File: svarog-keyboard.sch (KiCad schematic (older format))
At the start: 311 parts, among them J1 AVR-ISP-6, J10 I2C, J2 Conn_01x08_Male, J3 I2C, J4 I2C, J5 I2C, J6 I2C, J7 I2C, J8 I2C, J9 I2C, K1 KEYSW, K10 KEYSW, K11 KEYSW, K12 KEYSW, K13 KEYSW, K13-1 KEYSW, K14 KEYSW, K14-1 KEYSW, K14-2 KEYSW, K15 KEYSW, K16 KEYSW, K17 KEYSW, K18 KEYSW, K19 KEYSW, K2 KEYSW, K20 KEYSW, K21 KEYSW, K3 KEYSW, K4 KEYSW, K5 KEYSW, K6 KEYSW, K7 KEYSW, K8 KEYSW, K9 KEYSW, SW1 SW_BOOT, SW2 SW_RESET, U1 ATmega32A-PU, U2 MCP23017_SP, U3 MCP23017_SP, U4 MCP23017_SP, Y1 Crystal

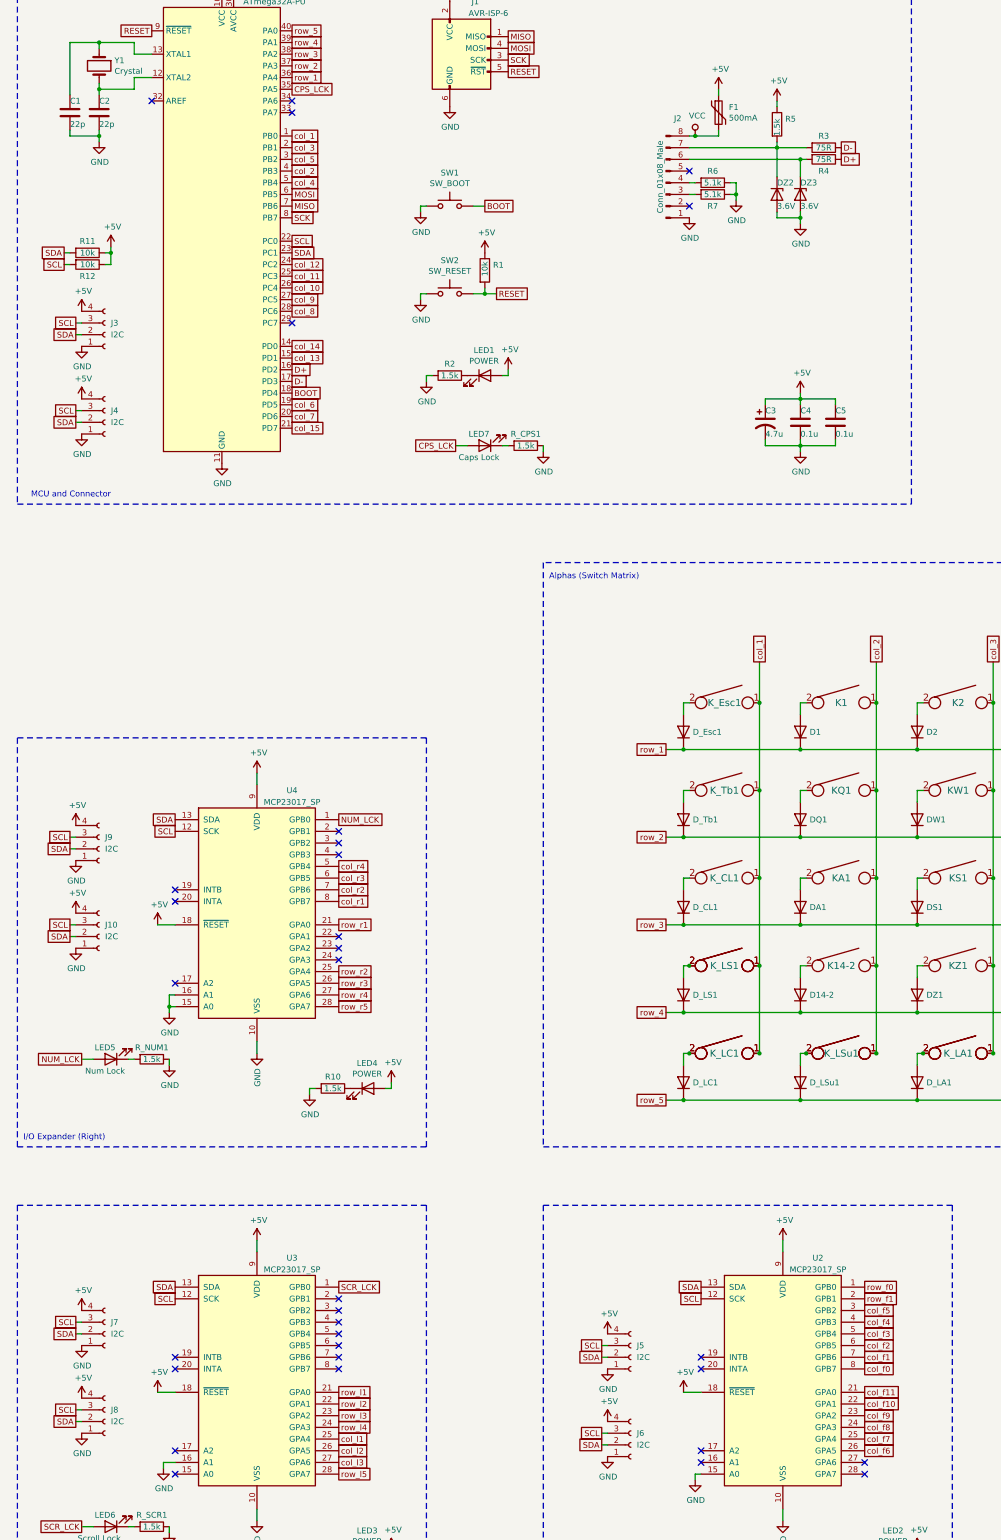
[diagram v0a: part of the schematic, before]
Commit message: Rev 0.1 [ALPHA] [UNTESTED]
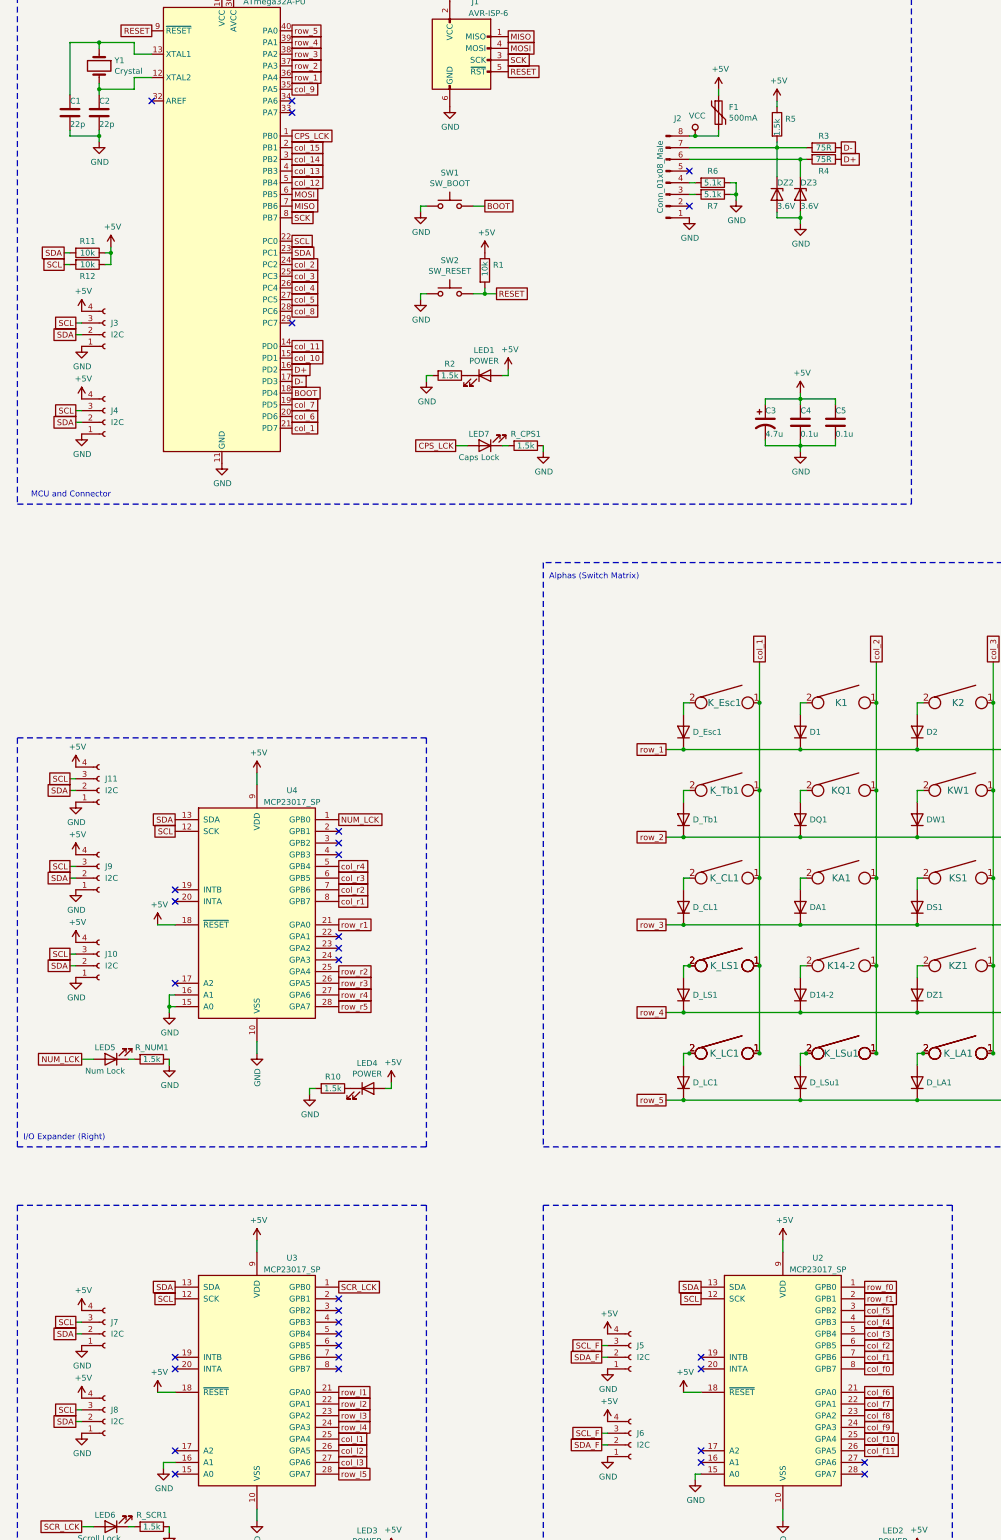
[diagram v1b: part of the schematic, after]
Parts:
- added J11: I2C, Connector_PinHeader_2.54mm:PinHeader_1x04_P2.54mm_Vertical, symbol Connector:Conn_01x04_Female
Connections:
- net +5V: now also J11.4 (Pin_4)
- net CPS_LCK: now also U1.1 (PB0); no longer U1.35 (PA5)
- net GND: now also J11.1 (Pin_1)
- net SCL: now also J11.3 (Pin_3); no longer J5.3 (Pin_3), J6.3 (Pin_3)
- net SDA: now also J11.2 (Pin_2); no longer J5.2 (Pin_2), J6.2 (Pin_2)
- net col_1: now also U1.21 (PD7); no longer U1.1 (PB0)
- net col_10: now also U1.15 (PD1); no longer U1.26 (PC4)
- net col_11: now also U1.14 (PD0); no longer U1.25 (PC3)
- net col_12: now also U1.5 (PB4); no longer U1.24 (PC2)
- net col_13: now also U1.4 (PB3); no longer U1.15 (PD1)
- net col_14: now also U1.3 (PB2); no longer U1.14 (PD0)
- net col_15: now also U1.2 (PB1); no longer U1.21 (PD7)
- net col_2: now also U1.24 (PC2); no longer U1.4 (PB3)
- net col_3: now also U1.25 (PC3); no longer U1.2 (PB1)
- net col_4: now also U1.26 (PC4); no longer U1.5 (PB4)
- net col_5: now also U1.27 (PC5); no longer U1.3 (PB2)
- net col_6: now also U1.20 (PD6); no longer U1.19 (PD5)
- net col_7: now also U1.19 (PD5); no longer U1.20 (PD6)
- net col_9: now also U1.35 (PA5); no longer U1.27 (PC5)
- net col_f10: now also U2.25 (GPA4); no longer U2.22 (GPA1)
- net col_f11: now also U2.26 (GPA5); no longer U2.21 (GPA0)
- net col_f6: now also U2.21 (GPA0); no longer U2.26 (GPA5)
- net col_f7: now also U2.22 (GPA1); no longer U2.25 (GPA4)
- net col_f8: now also U2.23 (GPA2); no longer U2.24 (GPA3)
- net col_f9: now also U2.24 (GPA3); no longer U2.23 (GPA2)
- new net SCL_F: J5.3 (Pin_3), J6.3 (Pin_3)
- new net SDA_F: J5.2 (Pin_2), J6.2 (Pin_2)
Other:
- moved on the sheet: J10, J9
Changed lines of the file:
@@
 Text GLabel 3350 1750 2    50   UnSpc ~ 0
 row_2
-Text GLabel 3350 2350 2    50   UnSpc ~ 0
+Text GLabel 3350 4850 2    50   UnSpc ~ 0
 col_1
-Text GLabel 3350 2450 2    50   UnSpc ~ 0
+Text GLabel 3350 3550 2    50   UnSpc ~ 0
 col_3
-Text GLabel 3350 2550 2    50   UnSpc ~ 0
+Text GLabel 3350 3750 2    50   UnSpc ~ 0
 col_5
 Text GLabel 3350 1450 2    50   UnSpc ~ 0
@@
 Text GLabel 3350 1850 2    50   UnSpc ~ 0
 row_1
+Text GLabel 3350 3450 2    50   UnSpc ~ 0
+col_2
+Text GLabel 3350 3650 2    50   UnSpc ~ 0
+col_4
+Text GLabel 3350 2550 2    50   UnSpc ~ 0
+col_14
 Text GLabel 3350 2650 2    50   UnSpc ~ 0
-col_2
+col_13
 Text GLabel 3350 2750 2    50   UnSpc ~ 0
-col_4
+col_12
 Text GLabel 3350 4150 2    50   UnSpc ~ 0
-col_14
+col_11
 Text GLabel 3350 4250 2    50   UnSpc ~ 0
-col_13
-Text GLabel 3350 3450 2    50   UnSpc ~ 0
-col_12
-Text GLabel 3350 3550 2    50   UnSpc ~ 0
-col_11
-Text GLabel 3350 3650 2    50   UnSpc ~ 0
 col_10
-Text GLabel 3350 3750 2    50   UnSpc ~ 0
+Text GLabel 3350 1950 2    50   UnSpc ~ 0
 col_9
 Text GLabel 3350 3850 2    50   UnSpc ~ 0
 col_8
+Text GLabel 3350 4650 2    50   UnSpc ~ 0
+col_7
+Text GLabel 3350 2450 2    50   UnSpc ~ 0
+col_15
 Text GLabel 3350 4750 2    50   UnSpc ~ 0
-col_7
-Text GLabel 3350 4850 2    50   UnSpc ~ 0
-col_15
-Text GLabel 3350 4650 2    50   UnSpc ~ 0
 col_6
 Wire Notes Line
@@
 Text GLabel 2350 8200 0    50   UnSpc ~ 0
 SDA
+Text GLabel 8250 13500 2    50   UnSpc ~ 0
+col_f10
+Text GLabel 8250 13600 2    50   UnSpc ~ 0
+col_f11
+Text GLabel 8250 13300 2    50   UnSpc ~ 0
+col_f8
+Text GLabel 8250 13400 2    50   UnSpc ~ 0
+col_f9
+Text GLabel 8250 13100 2    50   UnSpc ~ 0
+col_f6
 Text GLabel 8250 13200 2    50   UnSpc ~ 0
-col_f10
-Text GLabel 8250 13100 2    50   UnSpc ~ 0
-col_f11
-Text GLabel 8250 13400 2    50   UnSpc ~ 0
-col_f8
-Text GLabel 8250 13300 2    50   UnSpc ~ 0
-col_f9
-Text GLabel 8250 13600 2    50   UnSpc ~ 0
-col_f6
-Text GLabel 8250 13500 2    50   UnSpc ~ 0
 col_f7
 Text GLabel 8250 12500 2    50   UnSpc ~ 0
@@
 Wire Wire Line
 	1950 14250 2000 14250
-Text GLabel 3350 1950 2    50   UnSpc ~ 0
+Text GLabel 3350 2350 2    50   UnSpc ~ 0
 CPS_LCK
 Text GLabel 3750 8200 2    50   UnSpc ~ 0
@@
 $EndComp
 Text GLabel 6000 12800 0    50   UnSpc ~ 0
-SDA
+SDA_F
 Text GLabel 6000 12700 0    50   UnSpc ~ 0
-SCL
+SCL_F
 Wire Wire Line
 	6050 12700 6000 12700
@@
 	1    0    0    -1
 $EndComp
-Text GLabel 1450 8450 0    50   UnSpc ~ 0
+Text GLabel 1450 8700 0    50   UnSpc ~ 0
 SDA
-Text GLabel 1450 8350 0    50   UnSpc ~ 0
+Text GLabel 1450 8600 0    50   UnSpc ~ 0
 SCL
 Wire Wire Line
-	1500 8350 1450 8350
-Wire Wire Line
-	1500 8450 1450 8450
+	1500 8600 1450 8600
+Wire Wire Line
+	1500 8700 1450 8700
 $Comp
 L Connector:Conn_01x04_Female J9
 U 1 1 60AAE1B6
-P 1700 8450
-F 0 "J9" H 1750 8350 50  0000 L CNN
-F 1 "I2C" H 1750 8450 50  0000 L CNN
-F 2 "Connector_PinHeader_2.54mm:PinHeader_1x04_P2.54mm_Vertical" H 1700 8450 50  0001 C CNN
-F 3 "~" H 1700 8450 50  0001 C CNN
-	1    1700 8450
+P 1700 8700
+F 0 "J9" H 1750 8600 50  0000 L CNN
+F 1 "I2C" H 1750 8700 50  0000 L CNN
+F 2 "Connector_PinHeader_2.54mm:PinHeader_1x04_P2.54mm_Vertical" H 1700 8700 50  0001 C CNN
+F 3 "~" H 1700 8700 50  0001 C CNN
+	1    1700 8700
 	1    0    0    1
 $EndComp
@@
 L power:GND #PWR0152
 U 1 1 60AAE1BC
-P 1500 8550
-F 0 "#PWR0152" H 1500 8300 50  0001 C CNN
-F 1 "GND" H 1505 8377 50  0000 C CNN
-F 2 "" H 1500 8550 50  0001 C CNN
-F 3 "" H 1500 8550 50  0001 C CNN
-	1    1500 8550
+P 1500 8800
+F 0 "#PWR0152" H 1500 8550 50  0001 C CNN
+F 1 "GND" H 1505 8627 50  0000 C CNN
+F 2 "" H 1500 8800 50  0001 C CNN
+F 3 "" H 1500 8800 50  0001 C CNN
+	1    1500 8800
 	1    0    0    -1
 $EndComp
@@
 L power:+5V #PWR0153
 U 1 1 60AAE1C2
-P 1500 8250
-F 0 "#PWR0153" H 1500 8100 50  0001 C CNN
-F 1 "+5V" H 1515 8423 50  0000 C CNN
-F 2 "" H 1500 8250 50  0001 C CNN
-F 3 "" H 1500 8250 50  0001 C CNN
-	1    1500 8250
+P 1500 8500
+F 0 "#PWR0153" H 1500 8350 50  0001 C CNN
+F 1 "+5V" H 1515 8673 50  0000 C CNN
+F 2 "" H 1500 8500 50  0001 C CNN
+F 3 "" H 1500 8500 50  0001 C CNN
+	1    1500 8500
 	1    0    0    -1
 $EndComp
@@
 $EndComp
 Text GLabel 6000 13550 0    50   UnSpc ~ 0
-SDA
+SDA_F
 Text GLabel 6000 13450 0    50   UnSpc ~ 0
-SCL
+SCL_F
 Wire Wire Line
 	6050 13450 6000 13450
@@
 F 3 "" H 1550 13150 50  0001 C CNN
 	1    1550 13150
-	1    0    0    -1
-$EndComp
-Text GLabel 1450 9200 0    50   UnSpc ~ 0
-SDA
-Text GLabel 1450 9100 0    50   UnSpc ~ 0
-SCL
-Wire Wire Line
-	1500 9100 1450 9100
-Wire Wire Line
-	1500 9200 1450 9200
-$Comp
-L Connector:Conn_01x04_Female J10
-U 1 1 5E9D4282
-P 1700 9200
-F 0 "J10" H 1750 9100 50  0000 L CNN
-F 1 "I2C" H 1750 9200 50  0000 L CNN
-F 2 "Connector_PinHeader_2.54mm:PinHeader_1x04_P2.54mm_Vertical" H 1700 9200 50  0001 C CNN
-F 3 "~" H 1700 9200 50  0001 C CNN
-	1    1700 9200
-	1    0    0    1
-$EndComp
-$Comp
-L power:GND #PWR0161
-U 1 1 5E9D4288
-P 1500 9300
-F 0 "#PWR0161" H 1500 9050 50  0001 C CNN
-F 1 "GND" H 1505 9127 50  0000 C CNN
-F 2 "" H 1500 9300 50  0001 C CNN
-F 3 "" H 1500 9300 50  0001 C CNN
-	1    1500 9300
-	1    0    0    -1
-$EndComp
-$Comp
-L power:+5V #PWR0162
-U 1 1 5E9D428E
-P 1500 9000
-F 0 "#PWR0162" H 1500 8850 50  0001 C CNN
-F 1 "+5V" H 1515 9173 50  0000 C CNN
-F 2 "" H 1500 9000 50  0001 C CNN
-F 3 "" H 1500 9000 50  0001 C CNN
-	1    1500 9000
 	1    0    0    -1
 $EndComp
@@
 NoConn ~ 3750 8300
 NoConn ~ 3750 9200
+$Comp
+L power:+5V #PWR0162
+U 1 1 5E9D428E
+P 1500 9250
+F 0 "#PWR0162" H 1500 9100 50  0001 C CNN
+F 1 "+5V" H 1515 9423 50  0000 C CNN
+F 2 "" H 1500 9250 50  0001 C CNN
+F 3 "" H 1500 9250 50  0001 C CNN
+	1    1500 9250
+	1    0    0    -1
+$EndComp
+$Comp
+L power:GND #PWR0161
+U 1 1 5E9D4288
+P 1500 9550
+F 0 "#PWR0161" H 1500 9300 50  0001 C CNN
+F 1 "GND" H 1505 9377 50  0000 C CNN
+F 2 "" H 1500 9550 50  0001 C CNN
+F 3 "" H 1500 9550 50  0001 C CNN
+	1    1500 9550
+	1    0    0    -1
+$EndComp
+$Comp
+L Connector:Conn_01x04_Female J10
+U 1 1 5E9D4282
+P 1700 9450
+F 0 "J10" H 1750 9350 50  0000 L CNN
+F 1 "I2C" H 1750 9450 50  0000 L CNN
+F 2 "Connector_PinHeader_2.54mm:PinHeader_1x04_P2.54mm_Vertical" H 1700 9450 50  0001 C CNN
+F 3 "~" H 1700 9450 50  0001 C CNN
+	1    1700 9450
+	1    0    0    1
+$EndComp
+Wire Wire Line
+	1500 9450 1450 9450
+Wire Wire Line
+	1500 9350 1450 9350
+Text GLabel 1450 9350 0    50   UnSpc ~ 0
+SCL
+Text GLabel 1450 9450 0    50   UnSpc ~ 0
+SDA
+Text GLabel 1450 7950 0    50   UnSpc ~ 0
+SDA
+Text GLabel 1450 7850 0    50   UnSpc ~ 0
+SCL
+Wire Wire Line
+	1500 7850 1450 7850
+Wire Wire Line
+	1500 7950 1450 7950
+$Comp
+L Connector:Conn_01x04_Female J11
+U 1 1 5E3E2794
+P 1700 7950
+F 0 "J11" H 1750 7850 50  0000 L CNN
+F 1 "I2C" H 1750 7950 50  0000 L CNN
+F 2 "Connector_PinHeader_2.54mm:PinHeader_1x04_P2.54mm_Vertical" H 1700 7950 50  0001 C CNN
+F 3 "~" H 1700 7950 50  0001 C CNN
+	1    1700 7950
+	1    0    0    1
+$EndComp
+$Comp
+L power:GND #PWR0101
+U 1 1 5E3E279A
+P 1500 8050
+F 0 "#PWR0101" H 1500 7800 50  0001 C CNN
+F 1 "GND" H 1505 7877 50  0000 C CNN
+F 2 "" H 1500 8050 50  0001 C CNN
+F 3 "" H 1500 8050 50  0001 C CNN
+	1    1500 8050
+	1    0    0    -1
+$EndComp
+$Comp
+L power:+5V #PWR0102
+U 1 1 5E3E27A0
+P 1500 7750
+F 0 "#PWR0102" H 1500 7600 50  0001 C CNN
+F 1 "+5V" H 1515 7923 50  0000 C CNN
+F 2 "" H 1500 7750 50  0001 C CNN
+F 3 "" H 1500 7750 50  0001 C CNN
+	1    1500 7750
+	1    0    0    -1
+$EndComp
 $EndSCHEMATC
